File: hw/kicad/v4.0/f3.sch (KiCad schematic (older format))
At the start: 31 parts, among them P11 USB_OTG, P12 CONN_01X04, P7 CONN_01X03, T1 testpoint, T44 testpoint, T45 testpoint, T46 testpoint, U21 USBLC6-4SC6, U25 STM32F303CBTx, U29 USBLC6-4SC6, Y1 8M

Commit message: v4.0
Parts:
- D1: footprint LEDs:LED-0603 -> LEDs:LED-0805
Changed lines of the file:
@@
 F 0 "D1" H 17600 3800 50  0000 C CNN
 F 1 "LED" H 17600 3600 50  0000 C CNN
-F 2 "LEDs:LED-0603" H 17600 3700 50  0001 C CNN
+F 2 "LEDs:LED-0805" H 17600 3700 50  0001 C CNN
 F 3 "" H 17600 3700 50  0000 C CNN
 	1    17600 3700

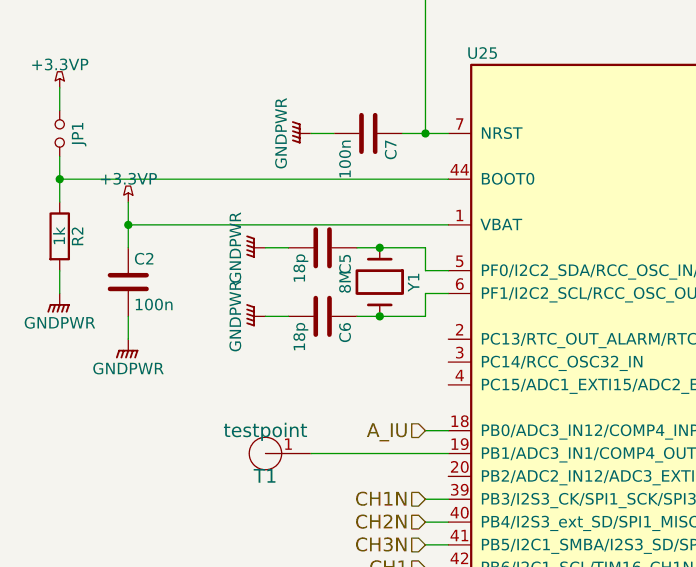
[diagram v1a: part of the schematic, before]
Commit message: v4.0
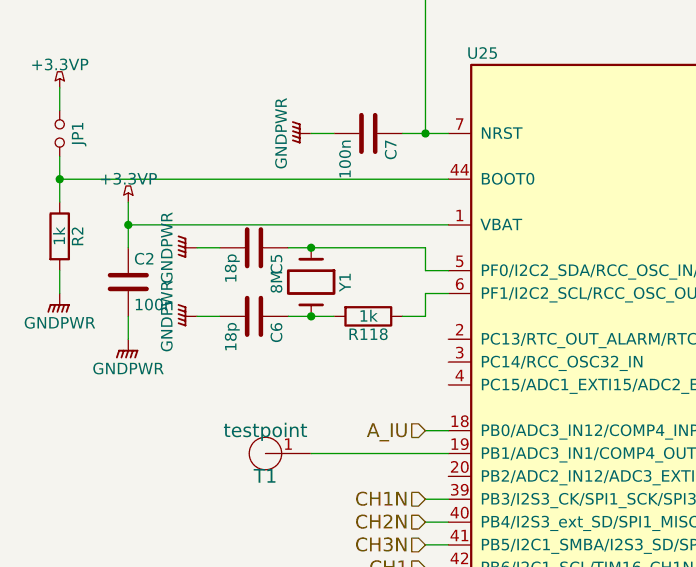
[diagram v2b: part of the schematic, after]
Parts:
- added R118: 1k, stmbl:R_0603, symbol R
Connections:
- net at C6.1, Y1.2: now also R118.2; no longer U25.6 (PF1/I2C2_SCL/RCC_OSC_OUT)
- new net: R118.1, U25.6 (PF1/I2C2_SCL/RCC_OSC_OUT)
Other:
- moved on the sheet: C5, C6, Y1
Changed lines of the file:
@@
 L Crystal Y1
 U 1 1 56631593
-P 2200 2250
-F 0 "Y1" H 2200 2400 50  0000 C CNN
-F 1 "8M" H 2200 2100 50  0000 C CNN
-F 2 "stmbl:Crystal_SMD_0603_4Pads" H 2200 2250 60  0001 C CNN
-F 3 "" H 2200 2250 60  0000 C CNN
-	1    2200 2250
+P 1900 2250
+F 0 "Y1" H 1900 2400 50  0000 C CNN
+F 1 "8M" H 1900 2100 50  0000 C CNN
+F 2 "stmbl:Crystal_SMD_0603_4Pads" H 1900 2250 60  0001 C CNN
+F 3 "" H 1900 2250 60  0000 C CNN
+	1    1900 2250
 	0    1    1    0
 $EndComp
@@
 L GNDPWR #PWR014
 U 1 1 566315E8
-P 1700 2100
-F 0 "#PWR014" H 1700 1900 50  0001 C CNN
-F 1 "GNDPWR" H 1700 1970 50  0000 C CNN
-F 2 "" H 1700 2050 60  0000 C CNN
-F 3 "" H 1700 2050 60  0000 C CNN
-	1    1700 2100
+P 1400 2100
+F 0 "#PWR014" H 1400 1900 50  0001 C CNN
+F 1 "GNDPWR" H 1400 1970 50  0000 C CNN
+F 2 "" H 1400 2050 60  0000 C CNN
+F 3 "" H 1400 2050 60  0000 C CNN
+	1    1400 2100
 	0    1    1    0
 $EndComp
@@
 L C C5
 U 1 1 56631605
-P 1950 2100
-F 0 "C5" H 1975 2200 50  0000 L CNN
-F 1 "18p" H 1975 2000 50  0000 L CNN
-F 2 "stmbl:C_0603" H 1988 1950 30  0001 C CNN
-F 3 "" H 1950 2100 60  0000 C CNN
-	1    1950 2100
+P 1650 2100
+F 0 "C5" H 1675 2200 50  0000 L CNN
+F 1 "18p" H 1675 2000 50  0000 L CNN
+F 2 "stmbl:C_0603" H 1688 1950 30  0001 C CNN
+F 3 "" H 1650 2100 60  0000 C CNN
+	1    1650 2100
 	0    1    1    0
 $EndComp
@@
 L GNDPWR #PWR015
 U 1 1 5663163A
-P 1700 2400
-F 0 "#PWR015" H 1700 2200 50  0001 C CNN
-F 1 "GNDPWR" H 1700 2270 50  0000 C CNN
-F 2 "" H 1700 2350 60  0000 C CNN
-F 3 "" H 1700 2350 60  0000 C CNN
-	1    1700 2400
+P 1400 2400
+F 0 "#PWR015" H 1400 2200 50  0001 C CNN
+F 1 "GNDPWR" H 1400 2270 50  0000 C CNN
+F 2 "" H 1400 2350 60  0000 C CNN
+F 3 "" H 1400 2350 60  0000 C CNN
+	1    1400 2400
 	0    1    1    0
 $EndComp
@@
 L C C6
 U 1 1 566316C7
-P 1950 2400
-F 0 "C6" H 1975 2500 50  0000 L CNN
-F 1 "18p" H 1975 2300 50  0000 L CNN
-F 2 "stmbl:C_0603" H 1988 2250 30  0001 C CNN
-F 3 "" H 1950 2400 60  0000 C CNN
-	1    1950 2400
+P 1650 2400
+F 0 "C6" H 1675 2500 50  0000 L CNN
+F 1 "18p" H 1675 2300 50  0000 L CNN
+F 2 "stmbl:C_0603" H 1688 2250 30  0001 C CNN
+F 3 "" H 1650 2400 60  0000 C CNN
+	1    1650 2400
 	0    1    1    0
 $EndComp
@@
 Wire Wire Line
 	1100 2000 2500 2000
-Connection ~ 2200 2100
+Connection ~ 1900 2100
 Wire Wire Line
 	2400 2100 2400 2200
 Wire Wire Line
 	2400 2200 2500 2200
-Connection ~ 2200 2400
+Connection ~ 1900 2400
 Wire Wire Line
 	2400 2300 2500 2300
@@
 	2400 2400 2400 2300
 Wire Wire Line
-	2100 2400 2400 2400
-Wire Wire Line
-	2100 2100 2400 2100
-Wire Wire Line
-	1700 2100 1800 2100
-Wire Wire Line
-	1700 2400 1800 2400
+	1800 2400 2000 2400
+Wire Wire Line
+	1800 2100 2400 2100
+Wire Wire Line
+	1400 2100 1500 2100
+Wire Wire Line
+	1400 2400 1500 2400
 Connection ~ 1100 2000
 Wire Wire Line
@@
 Wire Wire Line
 	2350 4400 2500 4400
+$Comp
+L R R118
+U 1 1 582CAB11
+P 2150 2400
+F 0 "R118" V 2230 2400 50  0000 C CNN
+F 1 "1k" V 2150 2400 50  0000 C CNN
+F 2 "stmbl:R_0603" V 2080 2400 30  0001 C CNN
+F 3 "" H 2150 2400 30  0000 C CNN
+	1    2150 2400
+	0    1    1    0
+$EndComp
+Wire Wire Line
+	2300 2400 2400 2400
 $EndSCHEMATC
